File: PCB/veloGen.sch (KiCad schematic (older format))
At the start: 42 parts, among them J1 CONN_01X02, J2 Gen. IN, J3 Batt, P1 TTL_232R_3V3, P2 CONN_01X04, Q1 STL4P3LLH6, Q2 BSS138_ok, U1 ESP-WROOM-32, U2 TS1101, U3 TS1101, U4 MAX8881

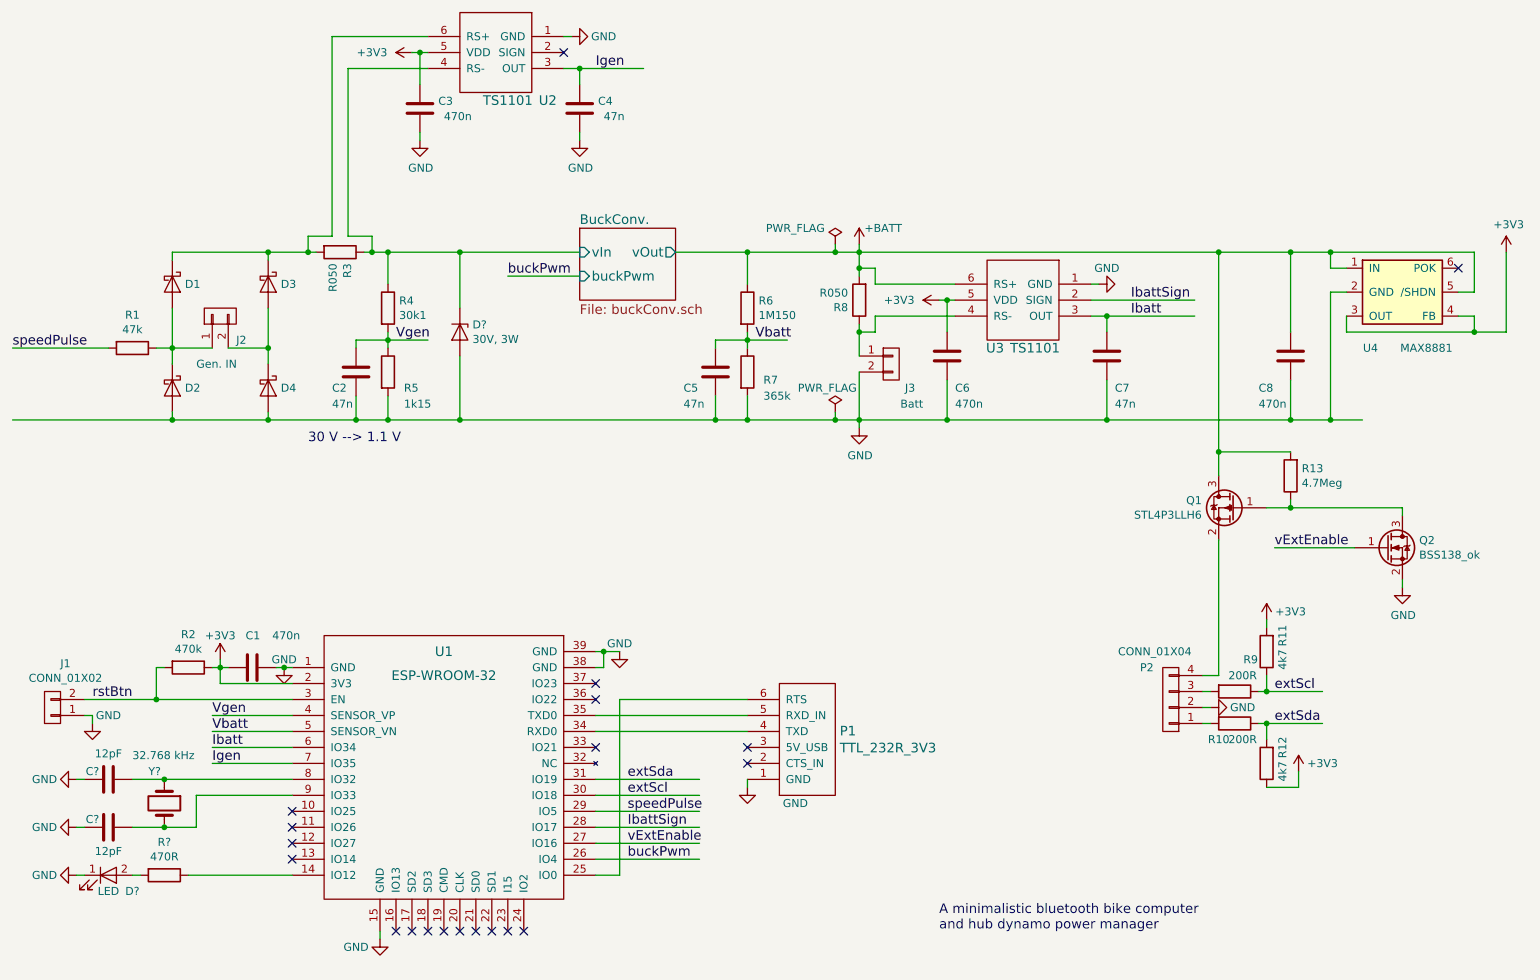
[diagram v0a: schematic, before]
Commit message: minor stuff:
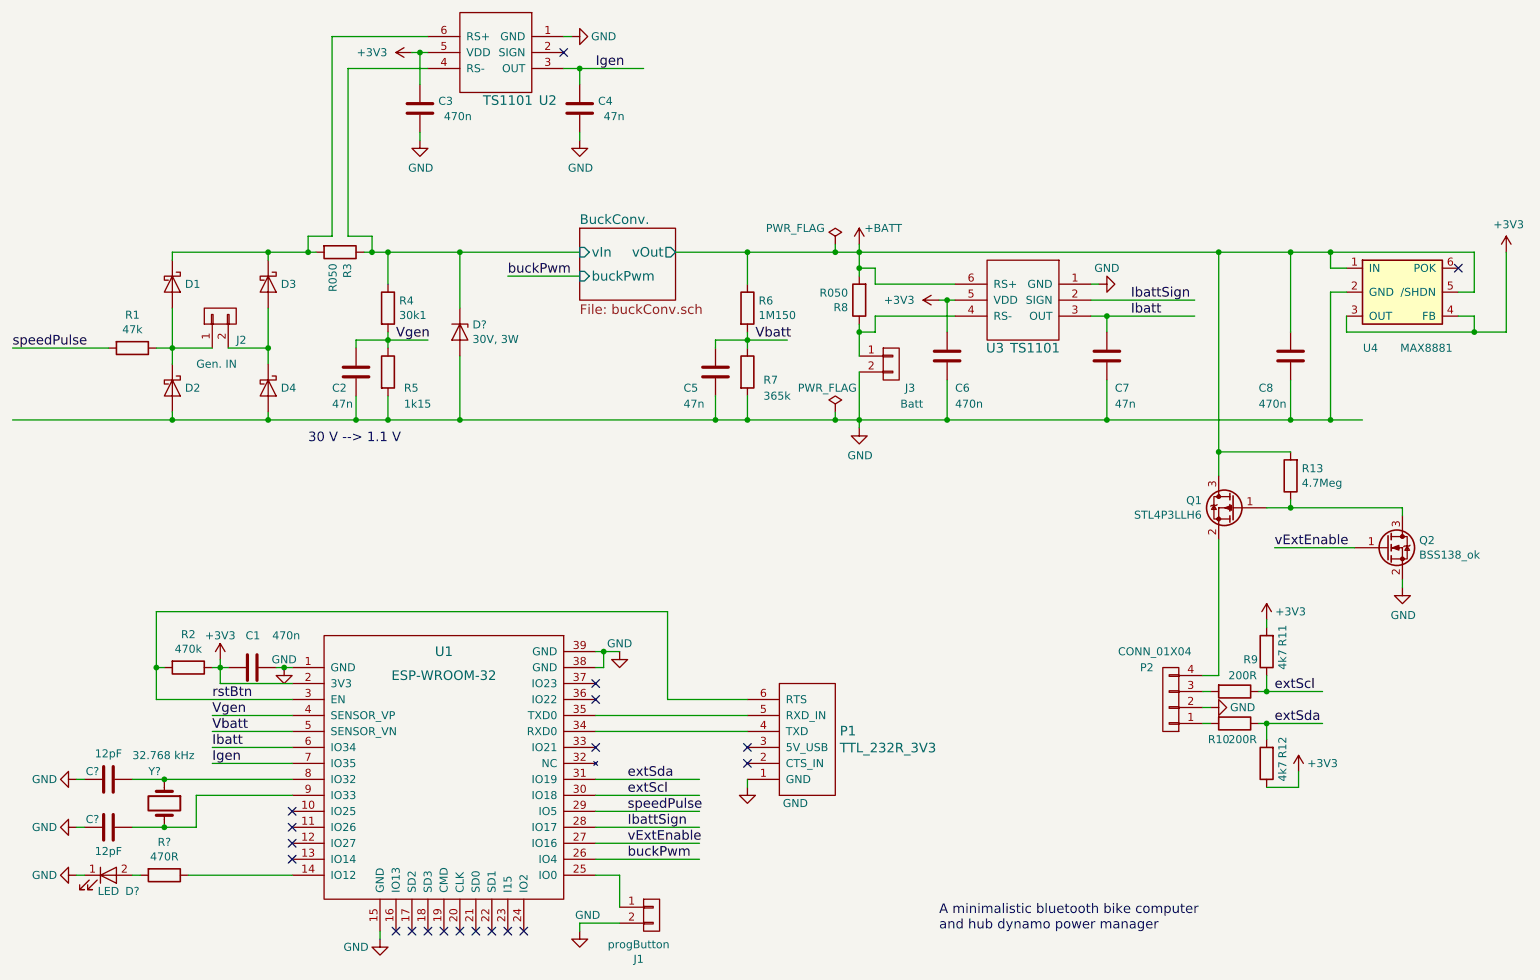
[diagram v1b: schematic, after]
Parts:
- J1: value CONN_01X02 -> progButton
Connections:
- wire segments 183 -> 134
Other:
- moved on the sheet: J1
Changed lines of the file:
@@
 	0    1    1    0
 $EndComp
-Text Label 1750 5300 0    60   ~ 0
+Text Label 2500 5300 0    60   ~ 0
 rstBtn
 $Comp
@@
 L CONN_01X02 J1
 U 1 1 58D2B56B
-P 1500 5350
-F 0 "J1" H 1419 5075 50  0000 C CNN
-F 1 "CONN_01X02" H 1419 5166 50  0000 C CNN
-F 2 "Pin_Headers:Pin_Header_Straight_1x02_Pitch2.54mm" H 1500 5350 50  0001 C CNN
-F 3 "" H 1500 5350 50  0001 C CNN
-	1    1500 5350
-	-1   0    0    1
+P 5250 6650
+F 0 "J1" H 5169 6375 50  0000 C CNN
+F 1 "progButton" H 5169 6466 50  0000 C CNN
+F 2 "Pin_Headers:Pin_Header_Straight_1x02_Pitch2.54mm" H 5250 6650 50  0001 C CNN
+F 3 "" H 5250 6650 50  0001 C CNN
+	1    5250 6650
+	1    0    0    -1
 $EndComp
 NoConn ~ 3000 6000
@@
 L GND #PWR1
 U 1 1 58D2F2FA
-P 1750 5450
-F 0 "#PWR1" H 1750 5200 50  0001 C CNN
-F 1 "GND" H 1850 5500 50  0000 C CNN
-F 2 "" H 1750 5450 50  0001 C CNN
-F 3 "" H 1750 5450 50  0001 C CNN
-	1    1750 5450
+P 4800 6750
+F 0 "#PWR1" H 4800 6500 50  0001 C CNN
+F 1 "GND" H 4850 6850 50  0000 C CNN
+F 2 "" H 4800 6750 50  0001 C CNN
+F 3 "" H 4800 6750 50  0001 C CNN
+	1    4800 6750
 	1    0    0    -1
 $EndComp
@@
 	3100 2400 3250 2400
 Wire Wire Line
-	2150 3100 2250 3100
-Wire Wire Line
-	2250 3100 2500 3100
-Wire Wire Line
-	2250 2850 2250 3100
-Wire Wire Line
-	2250 3100 2250 3200
+	2150 3100 2500 3100
+Wire Wire Line
+	2250 2850 2250 3200
 Connection ~ 2250 3100
 Wire Wire Line
 	2600 3100 2850 3100
 Wire Wire Line
-	2850 2850 2850 3100
-Wire Wire Line
-	2850 3100 2850 3200
+	2850 2850 2850 3200
 Connection ~ 2850 3100
 Wire Wire Line
@@
 	2250 3500 2250 3550
 Wire Wire Line
-	1250 3550 2250 3550
-Wire Wire Line
-	2250 3550 2850 3550
-Wire Wire Line
-	2850 3550 3400 3550
-Wire Wire Line
-	3400 3550 3600 3550
-Wire Wire Line
-	3600 3550 4050 3550
-Wire Wire Line
-	4050 3550 5650 3550
-Wire Wire Line
-	5650 3550 5850 3550
-Wire Wire Line
-	5850 3550 6400 3550
-Wire Wire Line
-	6400 3550 6550 3550
-Wire Wire Line
-	6550 3550 7100 3550
-Wire Wire Line
-	7100 3550 8100 3550
-Wire Wire Line
-	8100 3550 9250 3550
-Wire Wire Line
-	9250 3550 9500 3550
-Wire Wire Line
-	9500 3550 9700 3550
+	1250 3550 9700 3550
 Wire Wire Line
 	2850 3550 2850 3500
@@
 Connection ~ 2850 3550
 Wire Wire Line
-	5400 2500 5850 2500
-Wire Wire Line
-	5850 2500 6400 2500
-Wire Wire Line
-	6400 2500 6550 2500
-Wire Wire Line
-	6550 2500 8800 2500
-Wire Wire Line
-	8800 2500 9250 2500
-Wire Wire Line
-	9250 2500 9500 2500
-Wire Wire Line
-	9500 2500 10400 2500
-Wire Wire Line
-	6550 3250 6550 3550
-Wire Wire Line
-	6550 3550 6550 3600
-Wire Wire Line
-	6550 2950 6550 3000
-Wire Wire Line
-	6550 3000 6550 3150
-Wire Wire Line
-	6550 2450 6550 2500
-Wire Wire Line
-	6550 2500 6550 2600
-Wire Wire Line
-	6550 2600 6550 2650
+	5400 2500 10400 2500
+Wire Wire Line
+	6550 3250 6550 3600
+Wire Wire Line
+	6550 2950 6550 3150
+Wire Wire Line
+	6550 2450 6550 2650
 Connection ~ 6550 2500
 Connection ~ 6550 3550
@@
 Connection ~ 9250 2500
 Wire Wire Line
-	9600 3000 10400 3000
-Wire Wire Line
-	10400 3000 10600 3000
+	9600 3000 10600 3000
 Wire Wire Line
 	6650 2700 7150 2700
@@
 	6650 2900 7150 2900
 Wire Wire Line
-	7050 2800 7100 2800
-Wire Wire Line
-	7100 2800 7150 2800
+	7050 2800 7150 2800
 Wire Wire Line
 	7100 3000 7100 2800
@@
 	8050 2700 8000 2700
 Wire Wire Line
-	8000 2900 8100 2900
-Wire Wire Line
-	8100 2900 8650 2900
+	8000 2900 8650 2900
 Wire Wire Line
 	8000 2800 8650 2800
 Connection ~ 7100 3550
 Wire Wire Line
-	3750 1250 3800 1250
-Wire Wire Line
-	3800 1250 3850 1250
+	3750 1250 3850 1250
 Wire Wire Line
 	3800 1450 3800 1250
@@
 	4750 1150 4700 1150
 Wire Wire Line
-	4700 1350 4800 1350
-Wire Wire Line
-	4800 1350 5200 1350
+	4700 1350 5200 1350
 Wire Wire Line
 	3800 1800 3800 1750
@@
 	3600 3550 3600 3400
 Wire Wire Line
-	3600 3000 3600 3050
-Wire Wire Line
-	3600 3050 3600 3100
+	3600 3000 3600 3100
 Wire Wire Line
 	3400 3550 3400 3400
 Wire Wire Line
-	3400 3050 3600 3050
-Wire Wire Line
-	3600 3050 3850 3050
+	3400 3050 3850 3050
 Wire Wire Line
 	3400 3050 3400 3100
 Connection ~ 3600 3050
 Wire Wire Line
-	5850 3000 5850 3050
-Wire Wire Line
-	5850 3050 5850 3100
-Wire Wire Line
-	5650 3050 5850 3050
-Wire Wire Line
-	5850 3050 6100 3050
+	5850 3000 5850 3100
+Wire Wire Line
+	5650 3050 6100 3050
 Wire Wire Line
 	5650 3050 5650 3100
@@
 Connection ~ 5650 3550
 Wire Wire Line
-	2500 5100 2550 5100
-Wire Wire Line
-	2550 5100 2600 5100
+	2500 5100 2600 5100
 Wire Wire Line
 	2550 5200 3000 5200
 Wire Wire Line
-	2550 5050 2550 5100
-Wire Wire Line
-	2550 5100 2550 5200
+	2550 5050 2550 5200
 Connection ~ 2550 5100
 Wire Wire Line
-	2900 5100 2950 5100
-Wire Wire Line
-	2950 5100 3000 5100
+	2900 5100 3000 5100
 Connection ~ 2950 5100
 Wire Wire Line
-	4900 5000 4950 5000
-Wire Wire Line
-	4950 5000 5050 5000
+	4900 5000 5050 5000
 Wire Wire Line
 	4900 5100 4950 5100
@@
 	4350 2650 4800 2650
 Wire Wire Line
-	3450 2500 3500 2500
-Wire Wire Line
-	3500 2500 3600 2500
-Wire Wire Line
-	3600 2500 4050 2500
-Wire Wire Line
-	4050 2500 4800 2500
+	3450 2500 4800 2500
 Connection ~ 9500 3550
 Wire Wire Line
@@
 	10400 2500 10400 2750
 Wire Wire Line
-	8800 2500 8800 3750
-Wire Wire Line
-	8800 3750 8800 3900
+	8800 2500 8800 3900
 Connection ~ 8800 2500
 Wire Wire Line
@@
 Connection ~ 8800 3750
 Wire Wire Line
-	9100 4100 9250 4100
-Wire Wire Line
-	9250 4100 9950 4100
+	9100 4100 9950 4100
 Connection ~ 9250 4100
 Wire Wire Line
@@
 	8700 5250 8750 5250
 Wire Wire Line
-	9050 5250 9100 5250
-Wire Wire Line
-	9100 5250 9450 5250
-Wire Wire Line
-	9050 5450 9100 5450
-Wire Wire Line
-	9100 5450 9450 5450
+	9050 5250 9450 5250
+Wire Wire Line
+	9050 5450 9450 5450
 Wire Wire Line
 	9100 5550 9100 5450
@@
 Connection ~ 10400 3000
 Wire Wire Line
-	1700 5300 2150 5300
-Wire Wire Line
-	2150 5300 3000 5300
-Wire Wire Line
 	2200 5100 2150 5100
 Wire Wire Line
-	2150 5100 2150 5300
-Connection ~ 2150 5300
+	2150 4750 2150 5300
 Wire Wire Line
 	3000 5400 2500 5400
@@
 	4900 6400 5050 6400
 Wire Wire Line
-	5050 6400 5050 5300
-Wire Wire Line
-	5050 5300 5850 5300
-Wire Wire Line
 	5850 5400 4900 5400
 Wire Wire Line
@@
 	4900 5800 5550 5800
 Wire Wire Line
-	2250 2500 2850 2500
-Wire Wire Line
-	2850 2500 3100 2500
-Wire Wire Line
-	3100 2500 3150 2500
+	2250 2500 3150 2500
 Wire Wire Line
 	8750 5350 8700 5350
-Wire Wire Line
-	1700 5400 1750 5400
-Wire Wire Line
-	1750 5400 1750 5450
 Wire Wire Line
 	6400 2500 6400 2450
@@
 $EndComp
 Wire Wire Line
-	2000 5800 2200 5800
-Wire Wire Line
-	2200 5800 3000 5800
+	2000 5800 3000 5800
 Wire Wire Line
 	3000 5900 2400 5900
@@
 $EndComp
 Wire Wire Line
-	2400 6100 2200 6100
-Wire Wire Line
-	2200 6100 2000 6100
+	2400 6100 2000 6100
 Connection ~ 2200 5800
 Connection ~ 2200 6100
@@
 	1650 6400 1700 6400
 Connection ~ 2250 3550
+Wire Wire Line
+	2150 5300 3000 5300
+Wire Wire Line
+	5850 5300 5350 5300
+Wire Wire Line
+	5350 5300 5350 4750
+Wire Wire Line
+	5350 4750 2150 4750
+Connection ~ 2150 5100
+Wire Wire Line
+	5050 6400 5050 6600
+Wire Wire Line
+	5050 6700 4800 6700
+Wire Wire Line
+	4800 6700 4800 6750
 $EndSCHEMATC
